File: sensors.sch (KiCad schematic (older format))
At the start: 9 parts, among them J3 Screw_Terminal_01x08, J4 Screw_Terminal_01x08, J7 Screw_Terminal_01x02, J8 Conn_01x02_Male, U2 LTC2449CUHF, U4 INA126U

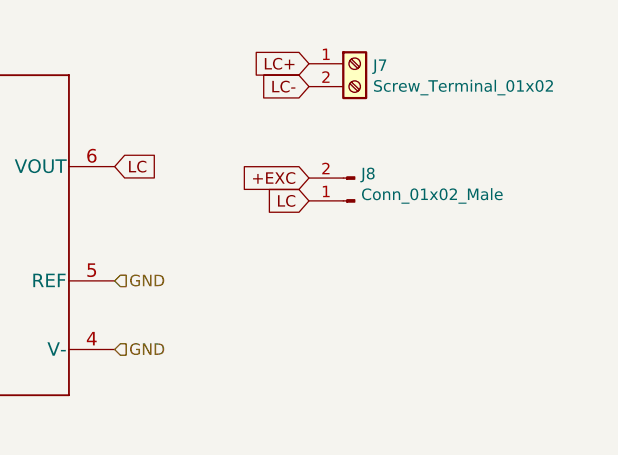
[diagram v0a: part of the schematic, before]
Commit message: completed design 2.0
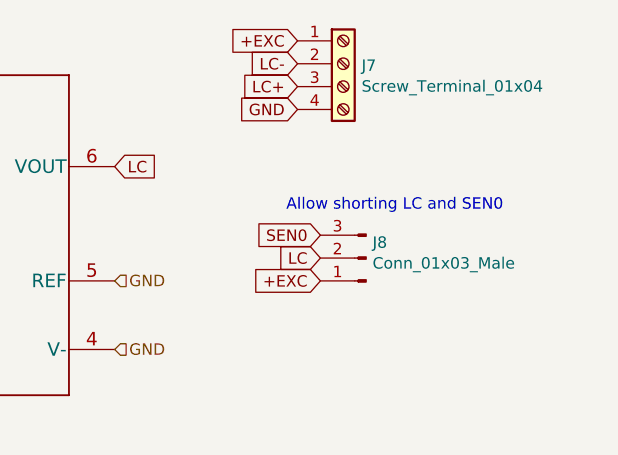
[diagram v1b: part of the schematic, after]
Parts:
- removed J7: Screw_Terminal_01x02, TerminalBlock_Phoenix:TerminalBlock_Phoenix_MKDS-1,5-2-5.08_1x02_P5.08mm_Horizontal, symbol Connector:Screw_Terminal_01x02
- removed J8: Conn_01x02_Male, Connector_PinHeader_2.54mm:PinHeader_1x02_P2.54mm_Vertical, symbol Connector:Conn_01x02_Male
- added J7: Screw_Terminal_01x04, TerminalBlock_Phoenix:TerminalBlock_Phoenix_MKDS-1,5-4-5.08_1x04_P5.08mm_Horizontal, symbol Connector:Screw_Terminal_01x04
- added J8: Conn_01x03_Male, Connector_PinHeader_2.54mm:PinHeader_1x03_P2.54mm_Vertical, symbol Connector:Conn_01x03_Male
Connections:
- net +EXC: now also J7.1 (Pin_1), J8.1 (Pin_1)
- net GND: now also J7.4 (Pin_4)
- net LC: now also J8.2 (Pin_2)
- net LC+: now also J7.3 (Pin_3)
- net LC-: now also J7.2 (Pin_2)
- net SEN0: now also J8.3 (Pin_3)
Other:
- note added: "Allow shorting LC and SEN0"
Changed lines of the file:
@@
 Text GLabel 7800 2400 0    50   Input ~ 0
 LC-
+Text GLabel 10000 1250 0    50   Input ~ 0
+LC+
+Text GLabel 10000 1150 0    50   Input ~ 0
+LC-
+Text GLabel 10100 2100 0    50   Input ~ 0
++EXC
+Text GLabel 10100 2000 0    50   Input ~ 0
+LC
 $Comp
-L Connector:Screw_Terminal_01x02 J7
-U 1 1 5EEF2437
-P 10250 1150
-F 0 "J7" H 10330 1142 50  0000 L CNN
-F 1 "Screw_Terminal_01x02" H 10330 1051 50  0000 L CNN
-F 2 "TerminalBlock_Phoenix:TerminalBlock_Phoenix_MKDS-1,5-2-5.08_1x02_P5.08mm_Horizontal" H 10250 1150 50  0001 C CNN
-F 3 "~" H 10250 1150 50  0001 C CNN
-	1    10250 1150
+L Connector:Conn_01x03_Male J8
+U 1 1 5EF5E577
+P 10300 2000
+F 0 "J8" H 10272 1932 50  0000 R CNN
+F 1 "Conn_01x03_Male" H 10272 2023 50  0000 R CNN
+F 2 "Connector_PinHeader_2.54mm:PinHeader_1x03_P2.54mm_Vertical" H 10300 2000 50  0001 C CNN
+F 3 "~" H 10300 2000 50  0001 C CNN
+	1    10300 2000
+	-1   0    0    1
+$EndComp
+Text GLabel 10100 1900 0    50   Input ~ 0
+SEN0
+Text Notes 10900 1800 2    50   ~ 0
+Allow shorting LC and SEN0
+$Comp
+L Connector:Screw_Terminal_01x04 J7
+U 1 1 5EF619ED
+P 10200 1150
+F 0 "J7" H 10280 1142 50  0000 L CNN
+F 1 "Screw_Terminal_01x04" H 10280 1051 50  0000 L CNN
+F 2 "TerminalBlock_Phoenix:TerminalBlock_Phoenix_MKDS-1,5-4-5.08_1x04_P5.08mm_Horizontal" H 10200 1150 50  0001 C CNN
+F 3 "~" H 10200 1150 50  0001 C CNN
+	1    10200 1150
 	1    0    0    -1
 $EndComp
-$Comp
-L Connector:Conn_01x02_Male J8
-U 1 1 5EEF4A47
-P 10250 1750
-F 0 "J8" H 10222 1632 50  0000 R CNN
-F 1 "Conn_01x02_Male" H 10222 1723 50  0000 R CNN
-F 2 "Connector_PinHeader_2.54mm:PinHeader_1x02_P2.54mm_Vertical" H 10250 1750 50  0001 C CNN
-F 3 "~" H 10250 1750 50  0001 C CNN
-	1    10250 1750
-	-1   0    0    1
-$EndComp
-Text GLabel 10050 1150 0    50   Input ~ 0
-LC+
-Text GLabel 10050 1250 0    50   Input ~ 0
-LC-
-Text GLabel 10050 1650 0    50   Input ~ 0
+Text GLabel 10000 1050 0    50   Input ~ 0
 +EXC
-Text GLabel 10050 1750 0    50   Input ~ 0
-LC
+Text GLabel 10000 1350 0    50   Input ~ 0
+GND
 $EndSCHEMATC
